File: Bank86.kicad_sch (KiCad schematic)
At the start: 1 part, among them U1 XCKU5P-FFVB676

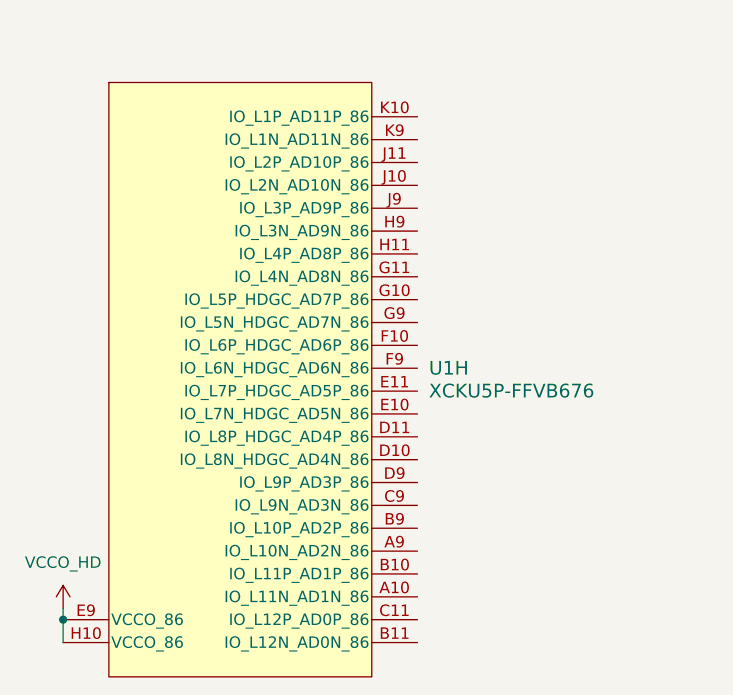
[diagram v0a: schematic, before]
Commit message: finishing schematic
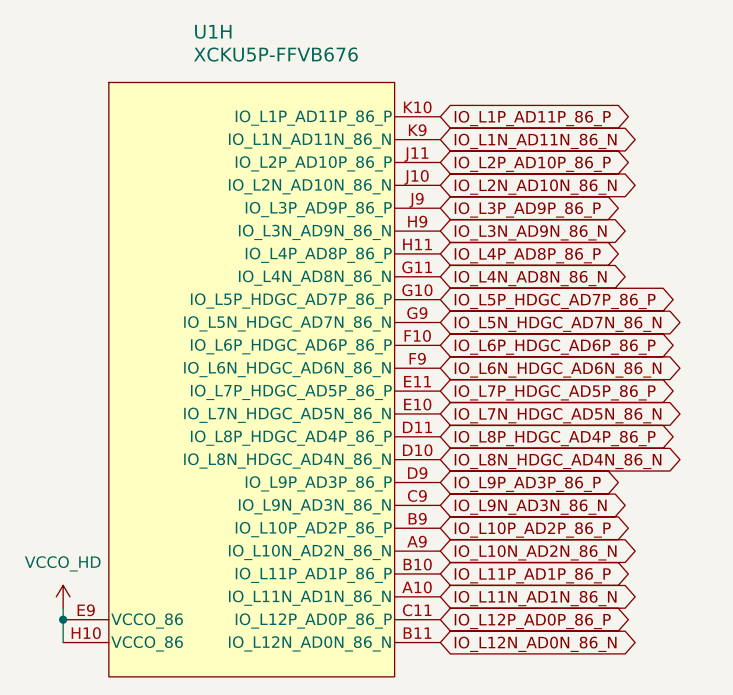
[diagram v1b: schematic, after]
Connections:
- net IO_L11N_AD1N_86_N: now reaches U1.A10 (IO_L11N_AD1N_86_N)
- net IO_L10N_AD2N_86_N: now reaches U1.A9 (IO_L10N_AD2N_86_N)
- net IO_L11P_AD1P_86_P: now reaches U1.B10 (IO_L11P_AD1P_86_P)
- net IO_L12N_AD0N_86_N: now reaches U1.B11 (IO_L12N_AD0N_86_N)
- net IO_L10P_AD2P_86_P: now reaches U1.B9 (IO_L10P_AD2P_86_P)
- net IO_L12P_AD0P_86_P: now reaches U1.C11 (IO_L12P_AD0P_86_P)
- net IO_L9N_AD3N_86_N: now reaches U1.C9 (IO_L9N_AD3N_86_N)
- net IO_L8N_HDGC_AD4N_86_N: now reaches U1.D10 (IO_L8N_HDGC_AD4N_86_N)
- net IO_L8P_HDGC_AD4P_86_P: now reaches U1.D11 (IO_L8P_HDGC_AD4P_86_P)
- net IO_L9P_AD3P_86_P: now reaches U1.D9 (IO_L9P_AD3P_86_P)
- net IO_L7N_HDGC_AD5N_86_N: now reaches U1.E10 (IO_L7N_HDGC_AD5N_86_N)
- net IO_L7P_HDGC_AD5P_86_P: now reaches U1.E11 (IO_L7P_HDGC_AD5P_86_P)
- net IO_L6P_HDGC_AD6P_86_P: now reaches U1.F10 (IO_L6P_HDGC_AD6P_86_P)
- net IO_L6N_HDGC_AD6N_86_N: now reaches U1.F9 (IO_L6N_HDGC_AD6N_86_N)
- net IO_L5P_HDGC_AD7P_86_P: now reaches U1.G10 (IO_L5P_HDGC_AD7P_86_P)
- net IO_L4N_AD8N_86_N: now reaches U1.G11 (IO_L4N_AD8N_86_N)
- net IO_L5N_HDGC_AD7N_86_N: now reaches U1.G9 (IO_L5N_HDGC_AD7N_86_N)
- net IO_L4P_AD8P_86_P: now reaches U1.H11 (IO_L4P_AD8P_86_P)
- net IO_L3N_AD9N_86_N: now reaches U1.H9 (IO_L3N_AD9N_86_N)
- net IO_L2N_AD10N_86_N: now reaches U1.J10 (IO_L2N_AD10N_86_N)
- net IO_L2P_AD10P_86_P: now reaches U1.J11 (IO_L2P_AD10P_86_P)
- net IO_L3P_AD9P_86_P: now reaches U1.J9 (IO_L3P_AD9P_86_P)
- net IO_L1P_AD11P_86_P: now reaches U1.K10 (IO_L1P_AD11P_86_P)
- net IO_L1N_AD11N_86_N: now reaches U1.K9 (IO_L1N_AD11N_86_N)
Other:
- moved on the sheet: U1H
